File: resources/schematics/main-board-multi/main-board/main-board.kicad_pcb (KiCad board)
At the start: 2 copper layers, 100 x 100 mm, 30 parts, among them J1 Conn_01x02_Female, J2 Conn_01x04_Female, J3 Conn_01x03_Female

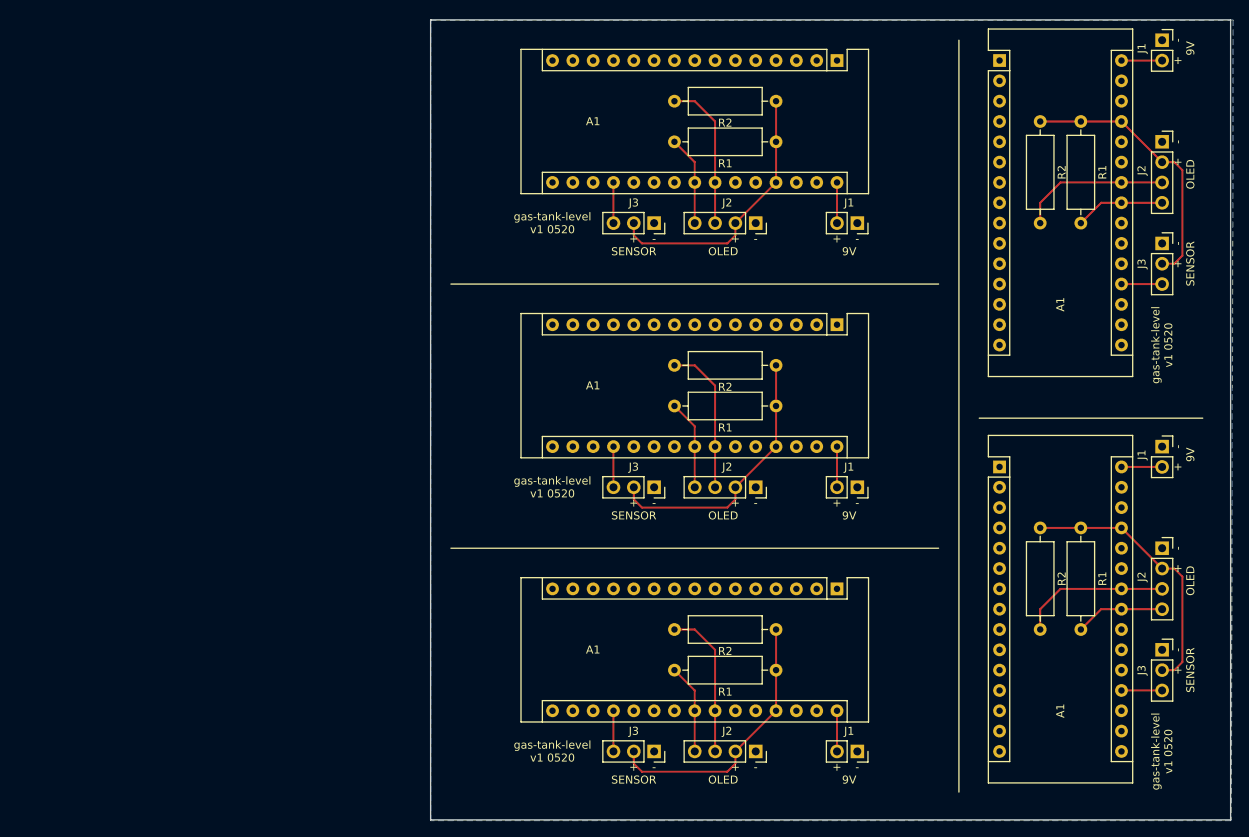
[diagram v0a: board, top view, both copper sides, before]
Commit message: Refactor PCB - batch-20201231
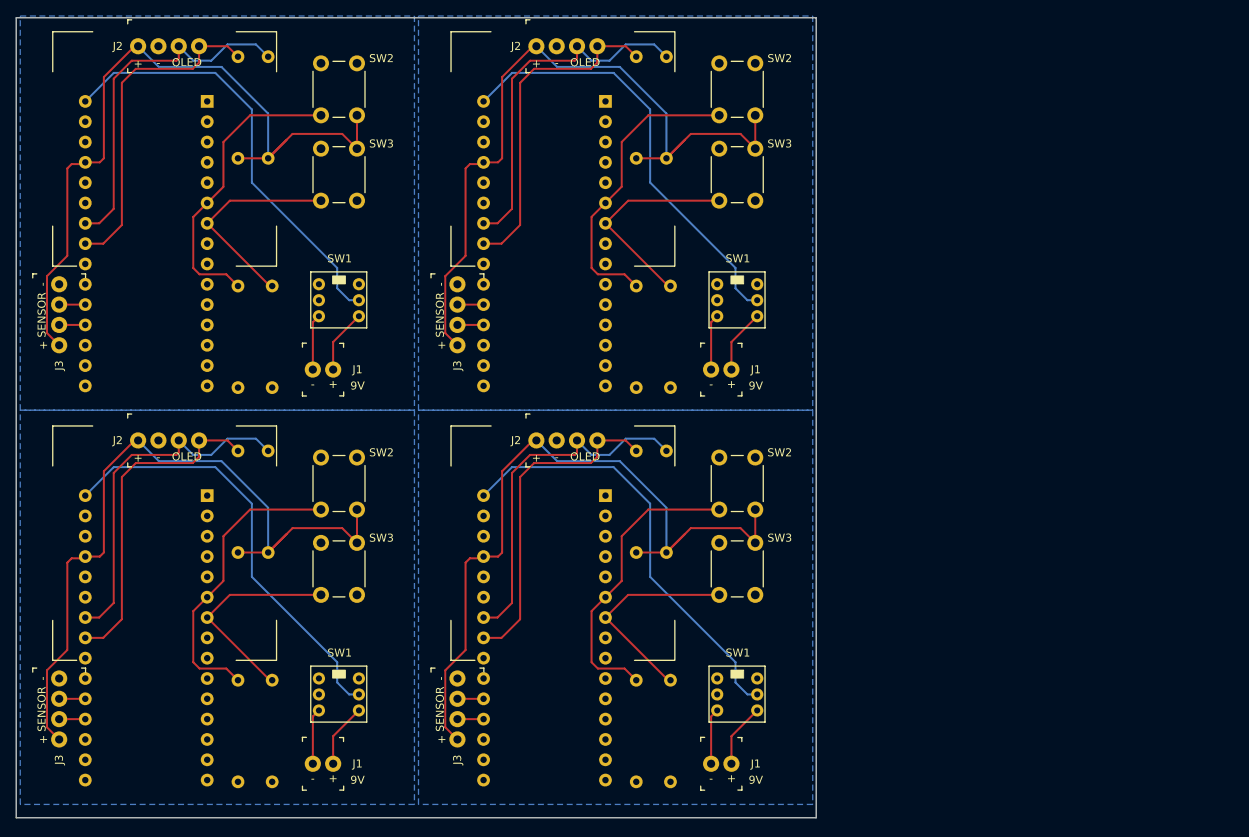
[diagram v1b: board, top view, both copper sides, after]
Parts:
- removed the A1 at (172.7, 106.7)
- removed the A1 at (172.7, 55.9)
- removed the A1 at (152.4, 121.9)
- removed the A1 at (152.4, 88.9)
- removed the A1 at (152.4, 55.9)
- removed the J1 at (193.0, 104.1)
- removed the J1 at (193.0, 53.3)
- removed the J1 at (154.9, 142.2)
- removed the J1 at (154.9, 109.2)
- removed the J2 at (193.0, 116.8)
- removed the J2 at (193.0, 66.0)
- removed the J2 at (142.2, 142.2)
- removed the J2 at (142.2, 109.2)
- removed the J2 at (142.2, 76.2)
- removed the J3 at (193.0, 129.5)
- removed the J3 at (193.0, 78.7)
- removed the J3 at (129.5, 142.2)
- removed the J3 at (129.5, 109.2)
- removed the J3 at (129.5, 76.2)
- removed the R1 at (182.9, 114.3)
- removed the R1 at (182.9, 63.5)
- removed the R1 at (144.8, 132.1)
- removed the R1 at (144.8, 99.1)
- removed the R2 at (177.8, 114.3)
- removed the R2 at (177.8, 63.5)
- removed the R2 at (144.8, 127.0)
- removed the R2 at (144.8, 94.0)
- added A1: Arduino_Nano_v3.x, Module:Arduino_Nano, B.Cu at (123.5, 110.3)
- added A1: Arduino_Nano_v3.x, Module:Arduino_Nano, B.Cu at (73.7, 110.3)
- added A1: Arduino_Nano_v3.x, Module:Arduino_Nano, B.Cu at (123.5, 61.0)
- added A1: Arduino_Nano_v3.x, Module:Arduino_Nano, B.Cu at (73.7, 61.0)
- added J1: Conn_01x02_Female, digikey-footprints:PinHeader_1x2_P2.54mm_Drill1.02mm, F.Cu at (136.7, 143.8)
- added J1: Conn_01x02_Female, digikey-footprints:PinHeader_1x2_P2.54mm_Drill1.02mm, F.Cu at (86.9, 143.8)
- added J1: Conn_01x02_Female, digikey-footprints:PinHeader_1x2_P2.54mm_Drill1.02mm, F.Cu at (136.7, 94.5)
- added J2: Conn_01x04_Female, digikey-footprints:PinHeader_1x4_P2.54mm_Drill1.02mm, F.Cu at (114.8, 103.4)
- added J2: Conn_01x04_Female, digikey-footprints:PinHeader_1x4_P2.54mm_Drill1.02mm, F.Cu at (65.0, 103.4)
- added J2: Conn_01x04_Female, digikey-footprints:PinHeader_1x4_P2.54mm_Drill1.02mm, F.Cu at (114.8, 54.1)
- added J2: Conn_01x04_Female, digikey-footprints:PinHeader_1x4_P2.54mm_Drill1.02mm, F.Cu at (65.0, 54.1)
- added J3: Conn_01x04_Female, digikey-footprints:PinHeader_1x4_P2.54mm_Drill1.02mm, F.Cu at (105.0, 133.1)
- added J3: Conn_01x04_Female, digikey-footprints:PinHeader_1x4_P2.54mm_Drill1.02mm, F.Cu at (55.2, 133.1)
- added J3: Conn_01x04_Female, digikey-footprints:PinHeader_1x4_P2.54mm_Drill1.02mm, F.Cu at (105.0, 83.8)
- added J3: Conn_01x04_Female, digikey-footprints:PinHeader_1x4_P2.54mm_Drill1.02mm, F.Cu at (55.2, 83.8)
- added R1: 3.3K, Resistor_THT:R_Axial_DIN0309_L9.0mm_D3.2mm_P12.70mm_Horizontal, B.Cu at (127.3, 117.4)
- added R1: 3.3K, Resistor_THT:R_Axial_DIN0309_L9.0mm_D3.2mm_P12.70mm_Horizontal, B.Cu at (77.5, 117.4)
- added R1: 3.3K, Resistor_THT:R_Axial_DIN0309_L9.0mm_D3.2mm_P12.70mm_Horizontal, B.Cu at (127.3, 68.1)
- added R2: 3.3K, Resistor_THT:R_Axial_DIN0309_L9.0mm_D3.2mm_P12.70mm_Horizontal, B.Cu at (81.3, 117.4)
- added R2: 3.3K, Resistor_THT:R_Axial_DIN0309_L9.0mm_D3.2mm_P12.70mm_Horizontal, B.Cu at (131.1, 117.4)
- added R2: 3.3K, Resistor_THT:R_Axial_DIN0309_L9.0mm_D3.2mm_P12.70mm_Horizontal, B.Cu at (131.1, 68.1)
- added R3: 10K, Resistor_THT:R_Axial_DIN0309_L9.0mm_D3.2mm_P12.70mm_Horizontal, B.Cu at (127.3, 146.0)
- added R3: 10K, Resistor_THT:R_Axial_DIN0309_L9.0mm_D3.2mm_P12.70mm_Horizontal, B.Cu at (77.5, 146.0)
- added R3: 10K, Resistor_THT:R_Axial_DIN0309_L9.0mm_D3.2mm_P12.70mm_Horizontal, B.Cu at (127.3, 96.8)
- added R3: 10K, Resistor_THT:R_Axial_DIN0309_L9.0mm_D3.2mm_P12.70mm_Horizontal, B.Cu at (77.5, 96.8)
- added R4: 10K, Resistor_THT:R_Axial_DIN0309_L9.0mm_D3.2mm_P12.70mm_Horizontal, B.Cu at (131.6, 146.0)
- added R4: 10K, Resistor_THT:R_Axial_DIN0309_L9.0mm_D3.2mm_P12.70mm_Horizontal, B.Cu at (81.8, 146.0)
- added R4: 10K, Resistor_THT:R_Axial_DIN0309_L9.0mm_D3.2mm_P12.70mm_Horizontal, B.Cu at (131.6, 96.8)
- added R4: 10K, Resistor_THT:R_Axial_DIN0309_L9.0mm_D3.2mm_P12.70mm_Horizontal, B.Cu at (81.8, 96.8)
- added SW1: SW_Push_DPDT, clvlabs:Switch_DPDT_7x7mm, F.Cu at (137.4, 133.1)
- added SW1: SW_Push_DPDT, clvlabs:Switch_DPDT_7x7mm, F.Cu at (87.6, 133.1)
- added SW1: SW_Push_DPDT, clvlabs:Switch_DPDT_7x7mm, F.Cu at (137.4, 83.8)
- added SW1: SW_Push_DPDT, clvlabs:Switch_DPDT_7x7mm, F.Cu at (87.6, 83.8)
- added SW2: SW_Push_45deg, Button_Switch_THT:SW_PUSH_6mm_H7.3mm, F.Cu at (137.7, 112.0)
- added SW2: SW_Push_45deg, Button_Switch_THT:SW_PUSH_6mm_H7.3mm, F.Cu at (87.9, 112.0)
- added SW2: SW_Push_45deg, Button_Switch_THT:SW_PUSH_6mm_H7.3mm, F.Cu at (137.7, 62.7)
- added SW2: SW_Push_45deg, Button_Switch_THT:SW_PUSH_6mm_H7.3mm, F.Cu at (87.9, 62.7)
- added SW3: SW_Push_45deg, Button_Switch_THT:SW_PUSH_6mm_H7.3mm, F.Cu at (137.7, 122.7)
- added SW3: SW_Push_45deg, Button_Switch_THT:SW_PUSH_6mm_H7.3mm, F.Cu at (87.9, 122.7)
- added SW3: SW_Push_45deg, Button_Switch_THT:SW_PUSH_6mm_H7.3mm, F.Cu at (137.7, 73.4)
- added SW3: SW_Push_45deg, Button_Switch_THT:SW_PUSH_6mm_H7.3mm, F.Cu at (87.9, 73.4)
- J1: footprint Connector_PinSocket_2.54mm:PinSocket_1x02_P2.54mm_Vertical -> digikey-footprints:PinHeader_1x2_P2.54mm_Drill1.02mm
- R1, R2: moved to B.Cu
- moved J1 70.5 mm to (86.9, 94.5), turned to 0 degrees
- moved R1 67.3 mm to (77.5, 68.1), turned to 90 degrees
- moved R2 63.9 mm to (81.3, 68.1), turned to 90 degrees
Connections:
- J1 pad 1: GND -> BATT_GND
- J1 pad 2: VIN -> BATT_VIN
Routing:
- net (no net): track 0.00 -> 968.9 mm
- net +5V: track 169.7 -> 94.6 mm
- net I2C_SCL: track 94.2 -> 45.2 mm
- net BUTTON_UP_PIN: track 0.00 -> 38.1 mm
- net VIN: track 25.4 -> 54.3 mm
- net BUTTON_DOWN_PIN: track 0.00 -> 27.5 mm
- net DISTANCE_SENSOR_PIN: track 25.4 -> 0.00 mm
- net I2C_SDA: track 56.1 -> 41.8 mm
- net BATT_VIN: track 0.00 -> 8.00 mm
- net BATT_GND: track 0.00 -> 6.98 mm
- net PING_TRIGGER_PIN: track 0.00 -> 3.26 mm
- net PING_ECHO_PIN: track 0.00 -> 3.26 mm
- added copper zone on B.Cu, net (none)
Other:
- rule pad_to_mask_clearance: 0.051 -> 0
- board text added: "20201231"
- board text added: "Arduino Nano"
- board text added: "github.com/clvLabs/gas-oil-tank-level"
- board text removed: "gas-tank-level v1 0520"
